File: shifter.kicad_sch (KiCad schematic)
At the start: 11 parts

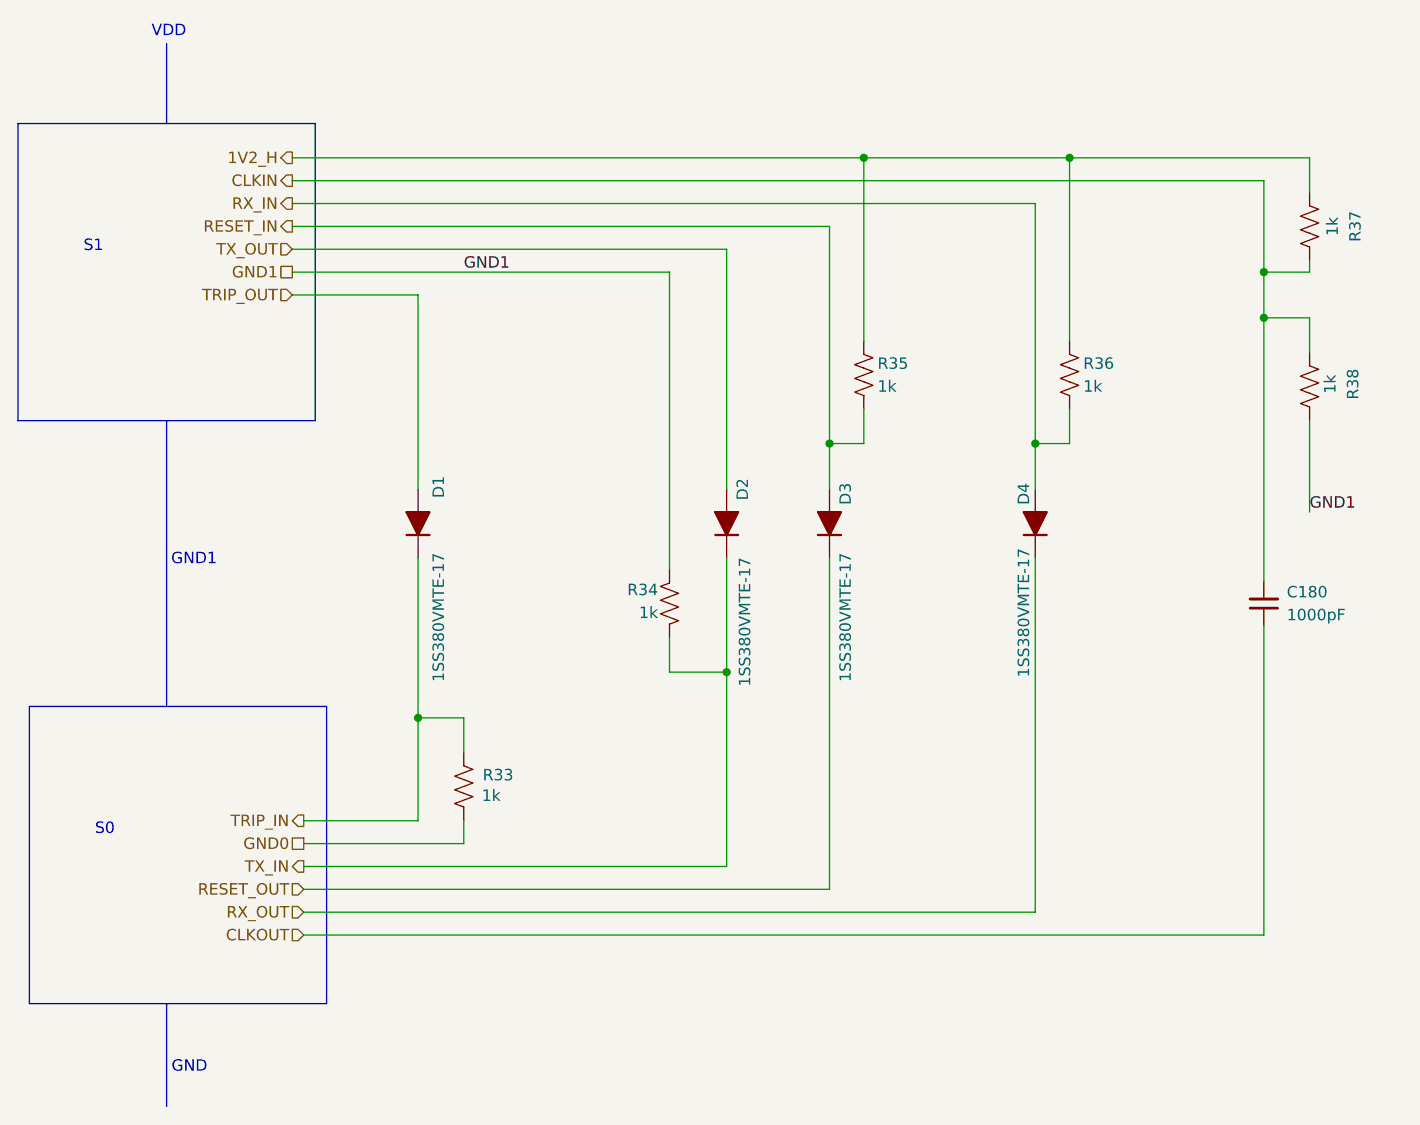
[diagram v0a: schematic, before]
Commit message: added gerbers and BOM
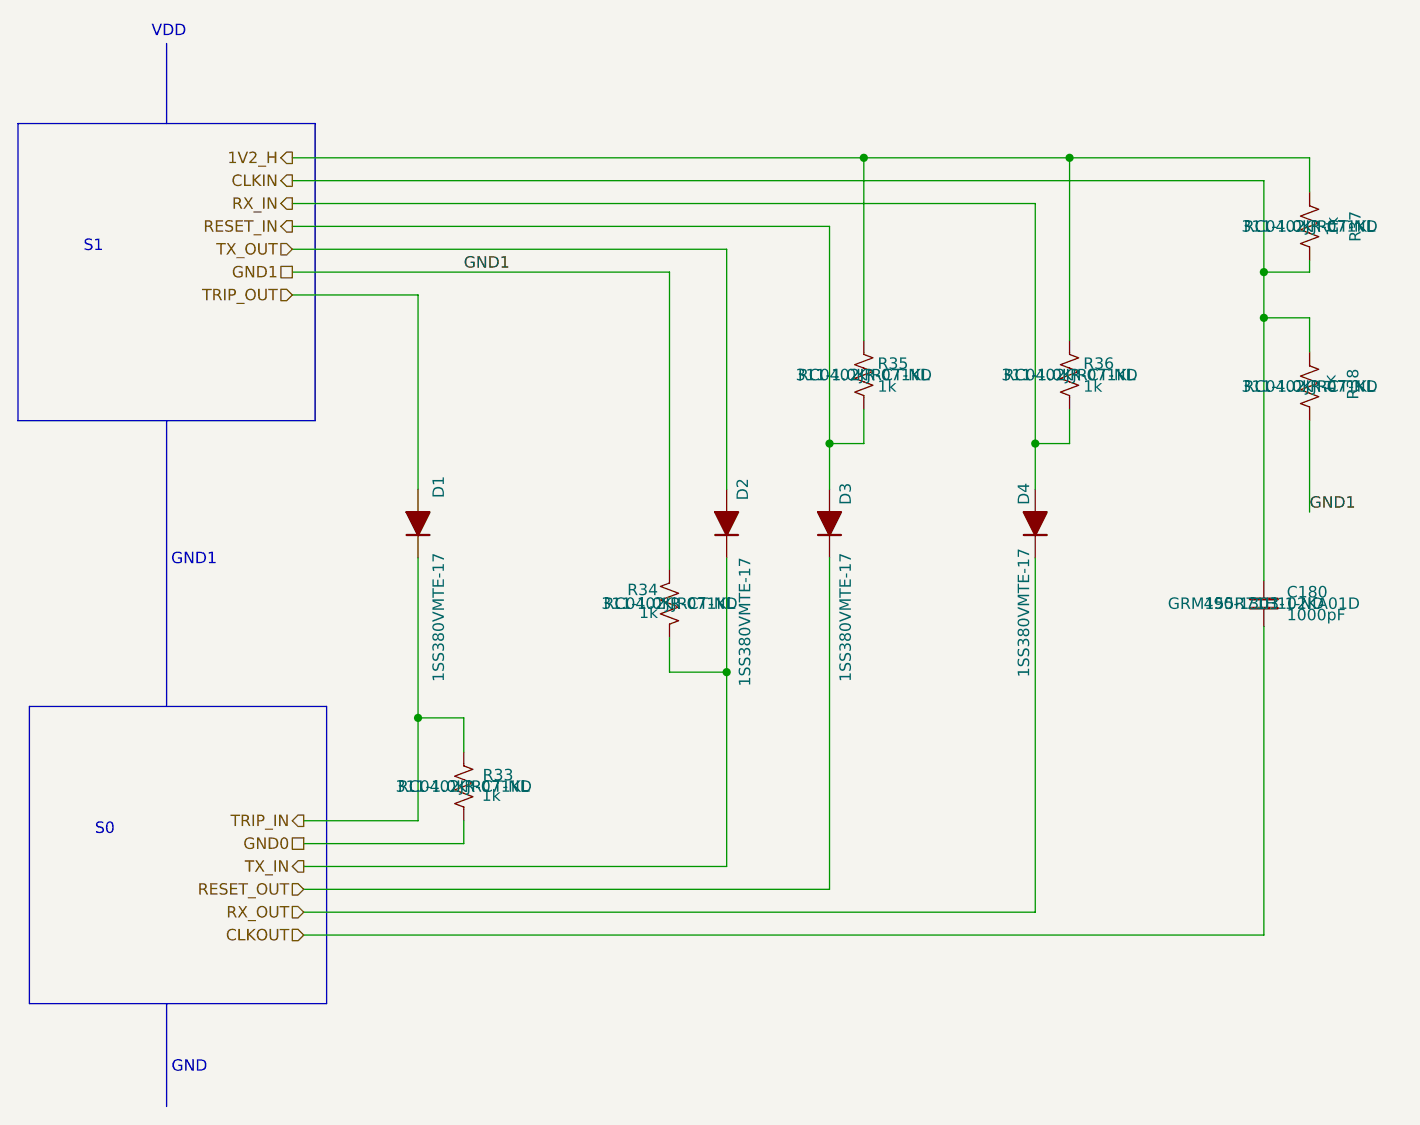
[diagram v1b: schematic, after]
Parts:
- C180: DK (none) -> 490-1303-1-ND; PARTNO (none) -> GRM155R71H102KA01D
- R33, R34, R35, R36, R37, R38: DK (none) -> 311-1.0KJRCT-ND; PARTNO (none) -> RC0402JR-071KL
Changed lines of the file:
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@@
+			)
+		)
+		(property "DK" "311-1.0KJRCT-ND"
+			(at 99.06 113.03 0)
+			(effects
+				(font
+					(size 1.27 1.27)
+				)
+			)
+		)
+		(property "PARTNO" "RC0402JR-071KL"
+			(at 99.06 113.03 0)
+			(effects
+				(font
+					(size 1.27 1.27)
+				)
 			)
 		)
@@
 			)
 		)
+		(property "DK" "490-1303-1-ND"
+			(at 187.96 92.71 0)
+			(effects
+				(font
+					(size 1.27 1.27)
+				)
+			)
+		)
+		(property "PARTNO" "GRM155R71H102KA01D"
+			(at 187.96 92.71 0)
+			(effects
+				(font
+					(size 1.27 1.27)
+				)
+			)
+		)
 		(pin "1"
 		)
@@
 				)
 				(hide yes)
+			)
+		)
+		(property "DK" "311-1.0KJRCT-ND"
+			(at 193.04 68.58 0)
+			(effects
+				(font
+					(size 1.27 1.27)
+				)
+			)
+		)
+		(property "PARTNO" "RC0402JR-071KL"
+			(at 193.04 68.58 0)
+			(effects
+				(font
+					(size 1.27 1.27)
+				)
 			)
 		)
@@
 			)
 		)
+		(property "DK" "311-1.0KJRCT-ND"
+			(at 121.92 92.71 0)
+			(effects
+				(font
+					(size 1.27 1.27)
+				)
+			)
+		)
+		(property "PARTNO" "RC0402JR-071KL"
+			(at 121.92 92.71 0)
+			(effects
+				(font
+					(size 1.27 1.27)
+				)
+			)
+		)
 		(pin "2"
 		)
@@
 			)
 		)
+		(property "DK" "311-1.0KJRCT-ND"
+			(at 143.51 67.31 0)
+			(effects
+				(font
+					(size 1.27 1.27)
+				)
+			)
+		)
+		(property "PARTNO" "RC0402JR-071KL"
+			(at 143.51 67.31 0)
+			(effects
+				(font
+					(size 1.27 1.27)
+				)
+			)
+		)
 		(pin "2"
 		)
@@
 			)
 		)
+		(property "DK" "311-1.0KJRCT-ND"
+			(at 166.37 67.31 0)
+			(effects
+				(font
+					(size 1.27 1.27)
+				)
+			)
+		)
+		(property "PARTNO" "RC0402JR-071KL"
+			(at 166.37 67.31 0)
+			(effects
+				(font
+					(size 1.27 1.27)
+				)
+			)
+		)
 		(pin "2"
 		)
@@
 			)
 		)
+		(property "DK" "311-1.0KJRCT-ND"
+			(at 193.04 50.8 0)
+			(effects
+				(font
+					(size 1.27 1.27)
+				)
+			)
+		)
+		(property "PARTNO" "RC0402JR-071KL"
+			(at 193.04 50.8 0)
+			(effects
+				(font
+					(size 1.27 1.27)
+				)
+			)
+		)
